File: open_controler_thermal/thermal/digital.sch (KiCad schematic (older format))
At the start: 55 parts, among them J1 Conn_01x02, J2 Conn_02x20_Odd_Even, J3 e_i_01x10, J4 e_i_02x10, J5 a_i_01x10

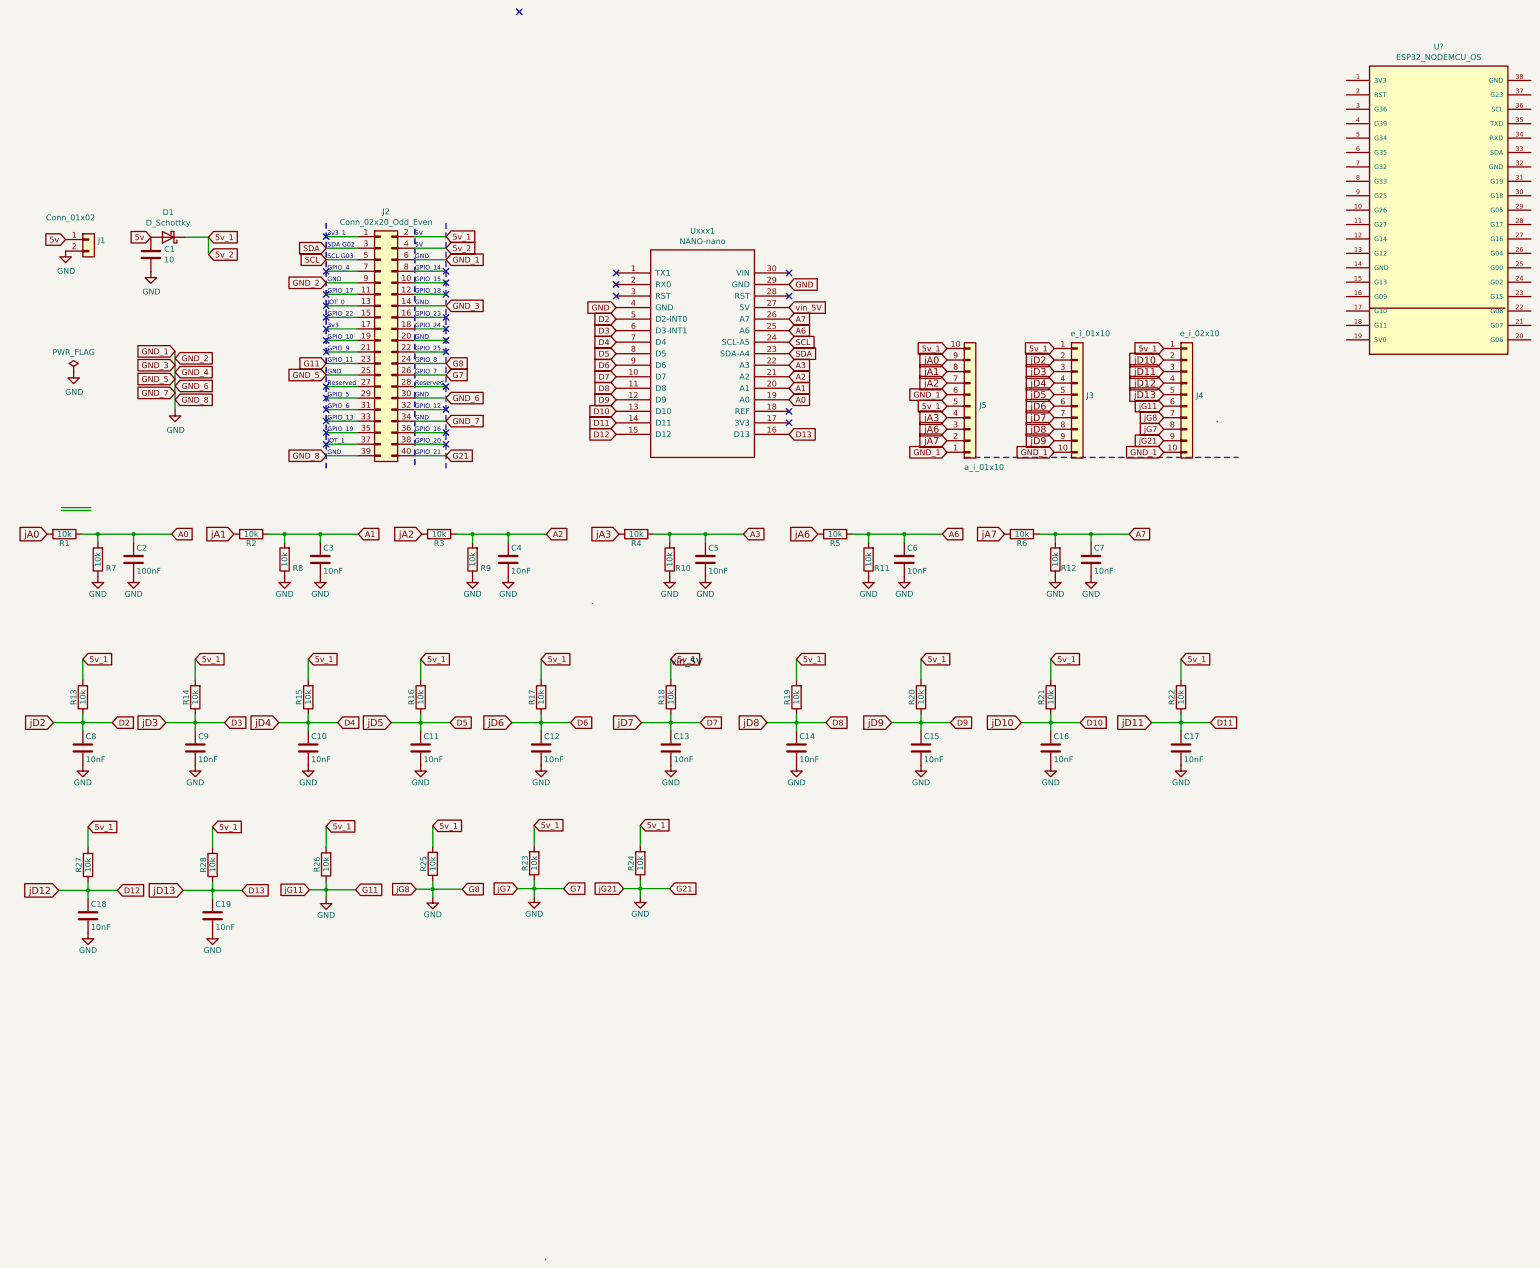
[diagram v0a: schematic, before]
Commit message: trabajando en openControllerDigital
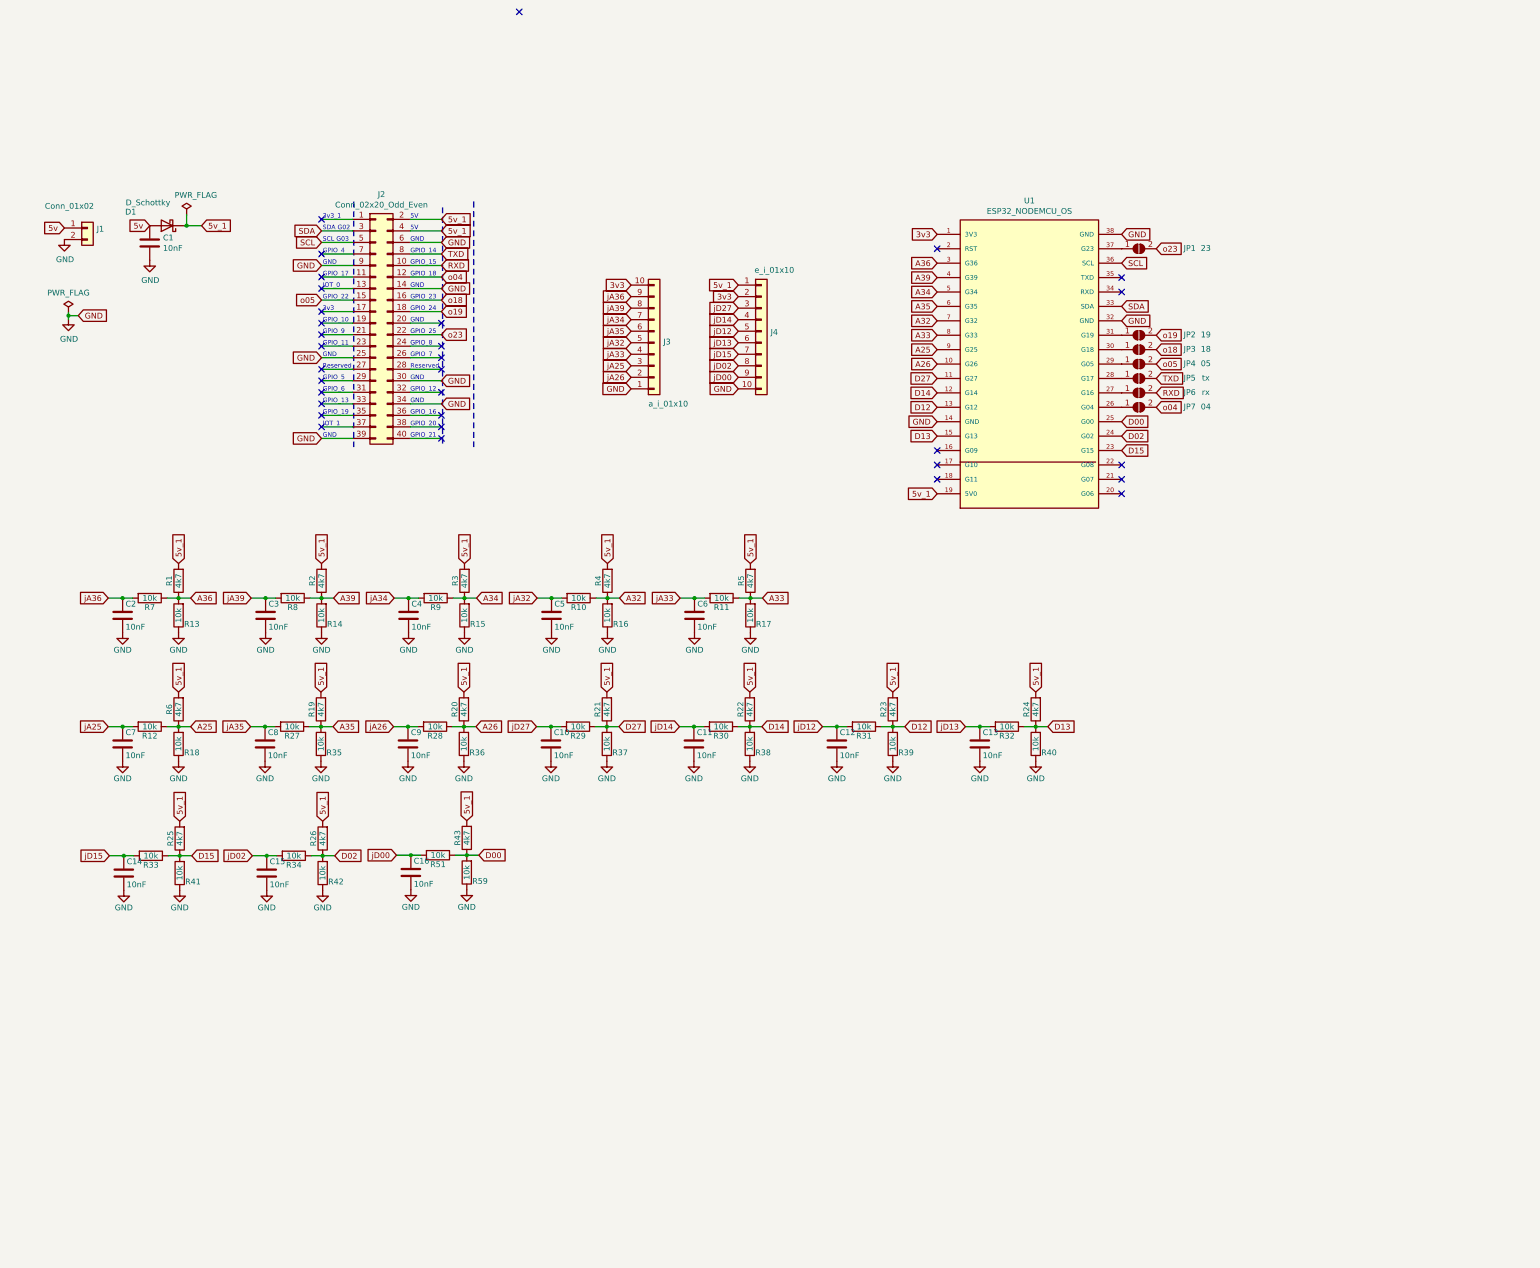
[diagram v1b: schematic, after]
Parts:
- removed C10, C11, C12, C13, C14, C15, C16, C17, C18, C19, C3, C4, C5, C6, C7, C8, C9: 10nF, eco_power_v2:C_1206_HandSoldering, symbol digital-rescue:C-wat-rescue
- removed C2: 100nF, eco_power_v2:C_1206_HandSoldering, symbol digital-rescue:C-wat-rescue
- removed J4: e_i_02x10, symbol Connector_Generic:Conn_01x10
- removed R1, R10, R11, R12, R13, R14, R15, R16, R17, R18, R19, R2, R20, R21, R22, R23, R24, R25, R26, R27, R28, R3, R4, R5, R6, R7, R8, R9: 10k, eco_power_v2:R_1206_HandSoldering, symbol digital-rescue:R-wat-rescue
- removed Uxxx1: NANO-nano, MODULE, symbol digital-rescue:NANO-nano-wat-rescue
- added C10, C11, C12, C13, C14, C15, C16, C2, C3, C4, C5, C6, C7, C8, C9: 10nF, Capacitor_SMD:C_1206_3216Metric_Pad1.42x1.75mm_HandSolder, symbol digital-rescue:C-wat-rescue-digital-rescue
- added JP1: 23, Jumper:SolderJumper-2_P1.3mm_Open_RoundedPad1.0x1.5mm, symbol Jumper:SolderJumper_2_Open
- added JP2: 19, Jumper:SolderJumper-2_P1.3mm_Open_RoundedPad1.0x1.5mm, symbol Jumper:SolderJumper_2_Open
- added JP3: 18, Jumper:SolderJumper-2_P1.3mm_Open_RoundedPad1.0x1.5mm, symbol Jumper:SolderJumper_2_Open
- added JP4: 05, Jumper:SolderJumper-2_P1.3mm_Open_RoundedPad1.0x1.5mm, symbol Jumper:SolderJumper_2_Open
- added JP5: tx, Jumper:SolderJumper-2_P1.3mm_Open_RoundedPad1.0x1.5mm, symbol Jumper:SolderJumper_2_Open
- added JP6: rx, Jumper:SolderJumper-2_P1.3mm_Open_RoundedPad1.0x1.5mm, symbol Jumper:SolderJumper_2_Open
- added JP7: 04, Jumper:SolderJumper-2_P1.3mm_Open_RoundedPad1.0x1.5mm, symbol Jumper:SolderJumper_2_Open
- added R1, R19, R2, R20, R21, R22, R23, R24, R25, R26, R3, R4, R43, R5, R6: 4k7, Resistor_SMD:R_1206_3216Metric_Pad1.42x1.75mm_HandSolder, symbol digital-rescue:R-wat-rescue-digital-rescue
- added R10, R11, R12, R13, R14, R15, R16, R17, R18, R27, R28, R29, R30, R31, R32, R33, R34, R35, R36, R37, R38, R39, R40, R41, R42, R51, R59, R7, R8, R9: 10k, Resistor_SMD:R_1206_3216Metric_Pad1.42x1.75mm_HandSolder, symbol digital-rescue:R-wat-rescue-digital-rescue
- C1: value 10 -> 10nF; footprint (none) -> Capacitor_SMD:C_1206_3216Metric_Pad1.42x1.75mm_HandSolder
- D1: footprint (none) -> Digital:D_2114_3652Metric
- J1: footprint (none) -> Connector_Phoenix_MC:PhoenixContact_MCV_1,5_2-G-3.5_1x02_P3.50mm_Vertical
- J2: footprint (none) -> Connector_PinHeader_2.54mm:PinHeader_2x20_P2.54mm_Vertical
- J3: renamed from J5; footprint (none) -> Connector_Phoenix_MC:PhoenixContact_MCV_1,5_10-G-3.5_1x10_P3.50mm_Vertical
- J4: renamed from J3; footprint (none) -> Connector_Phoenix_MC:PhoenixContact_MCV_1,5_10-G-3.5_1x10_P3.50mm_Vertical
- U1: renamed from U?; footprint ESP32 -> Espressif:ESP32-DevKitC
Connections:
- net D2 is gone; now on net 3v3: J4.2 (Pin_2)
- net 5v_1: now also U1.19 (5V0), R1.2, R19.2, R2.2, R20.2, R21.2, R22.2, R23.2, R24.2, R25.2, R26.2, R3.2, R4.2, R43.2, R5.2, R6.2; no longer J3.10 (Pin_10), J3.5 (Pin_5)
- net D12: now also U1.13 (G12), R23.1, R31.1, R39.2
- net D13: now also U1.15 (G13), R24.1, R32.1, R40.2
- net GND: now also U1.14 (GND), U1.32 (GND), U1.38 (GND), C10.2, C11.2, C12.2, C13.2, C14.2, C15.2, C16.2, C2.2, C3.2, C4.2, C5.2, C6.2, C7.2, C8.2, C9.2, R13.1, R14.1, R15.1, R16.1, R17.1, R18.1, R35.1, R36.1, R37.1, R38.1, R39.1, R40.1, R41.1, R42.1, R59.1; no longer J2.23 (Pin_23), J2.24 (Pin_24), J2.26 (Pin_26), J2.40 (Pin_40), J3.6 (Pin_6)
- net SCL: now also U1.36 (SCL)
- net SDA: now also U1.33 (SDA)
- net RXD: now reaches J2.10 (Pin_10)
- net RXD: now also JP6.2 (B)
- net o04: now reaches J2.12 (Pin_12)
- net o04: now also JP7.2 (B)
- net o05: now reaches J2.15 (Pin_15)
- net o05: now also JP4.2 (B)
- net o18: now reaches J2.16 (Pin_16)
- net o18: now also JP3.2 (B)
- net o19: now reaches J2.18 (Pin_18)
- net o19: now also JP2.2 (B)
- net o23: now reaches J2.22 (Pin_22)
- net o23: now also JP1.2 (B)
- net TXD: now reaches J2.8 (Pin_8)
- net TXD: now also JP5.2 (B)
- net 3v3: now reaches U1.1 (3V3)
- net 3v3: now also J3.10 (Pin_10)
- net A26: now reaches U1.10 (G26)
- net A26: now also R20.1, R28.1, R36.2
- net D27: now reaches U1.11 (G27)
- net D27: now also R21.1, R29.1, R37.2
- net D14: now reaches U1.12 (G14)
- net D14: now also R22.1, R30.1, R38.2
- net D15: now reaches U1.23 (G15)
- net D15: now also R25.1, R33.1, R41.2
- net D02: now reaches U1.24 (G02)
- net D02: now also R26.1, R34.1, R42.2
- net D00: now reaches U1.25 (G00)
- net D00: now also R43.1, R51.1, R59.2
- net at U1.26 (G04): now also JP7.1 (A)
- net at U1.27 (G16): now also JP6.1 (A)
- net at U1.28 (G17): now also JP5.1 (A)
- net at U1.29 (G05): now also JP4.1 (A)
- net A36: now reaches U1.3 (G36)
- net A36: now also R1.1, R13.2, R7.1
- net at U1.30 (G18): now also JP3.1 (A)
- net at U1.31 (G19): now also JP2.1 (A)
- net at U1.37 (G23): now also JP1.1 (A)
- net A39: now reaches U1.4 (G39)
- net A39: now also R14.2, R2.1, R8.1
- net A34: now reaches U1.5 (G34)
- net A34: now also R15.2, R3.1, R9.1
- net A35: now reaches U1.6 (G35)
- net A35: now also R19.1, R27.1, R35.2
- net A32: now reaches U1.7 (G32)
- net A32: now also R10.1, R16.2, R4.1
- net A33: now reaches U1.8 (G33)
- net A33: now also R11.1, R17.2, R5.1
- net A25: now reaches U1.9 (G25)
- net A25: now also R12.1, R18.2, R6.1
- net D3 renamed jD27
- net jD27: now also C10.1, R29.2
- net D4 renamed jD14
- net jD14: now also C11.1, R30.2
- net D5 renamed jD12
- net jD12: now also C12.1, R31.2
- net D6 renamed jD13
- net jD13: now also C13.1, R32.2
- net D7 renamed jD15
- net jD15: now also C14.1, R33.2
- net D8 renamed jD02
- net jD02: now also C15.1, R34.2
- net D9 renamed jD00
- net jD00: now also C16.1, R51.2
- net jA0 renamed jA36
- net jA36: now also C2.1, R7.2
- net jA1 renamed jA39
- net jA39: now also C3.1, R8.2
- net jA2 renamed jA34
- net jA34: now also C4.1, R9.2
- net jA3 renamed jA33
- net jA33: now also C6.1, R11.2
- net jA6 renamed jA25
- net jA25: now also C7.1, R12.2
- net jA7 renamed jA26
- net jA26: now also C9.1, R28.2
- new net jA32: C5.1, J3.5 (Pin_5), R10.2
- new net jA35: C8.1, J3.6 (Pin_6), R27.2
- no-connect marks 33 -> 32
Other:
- moved on the sheet: C1, D1, J1, J2, J3, J4, U1
